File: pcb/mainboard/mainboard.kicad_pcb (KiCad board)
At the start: 2 copper layers, 100 x 100 mm, 50 parts, among them J2 SWD, J3 Conn_01x10, J4 M1, J5 M2, K1 SANYOU_SRD_Form_C, SW1 RES_BUT, SW2 BOOT_SW, U1 STM32G474RETx, U5 INA219AxD, Y1 16MHz

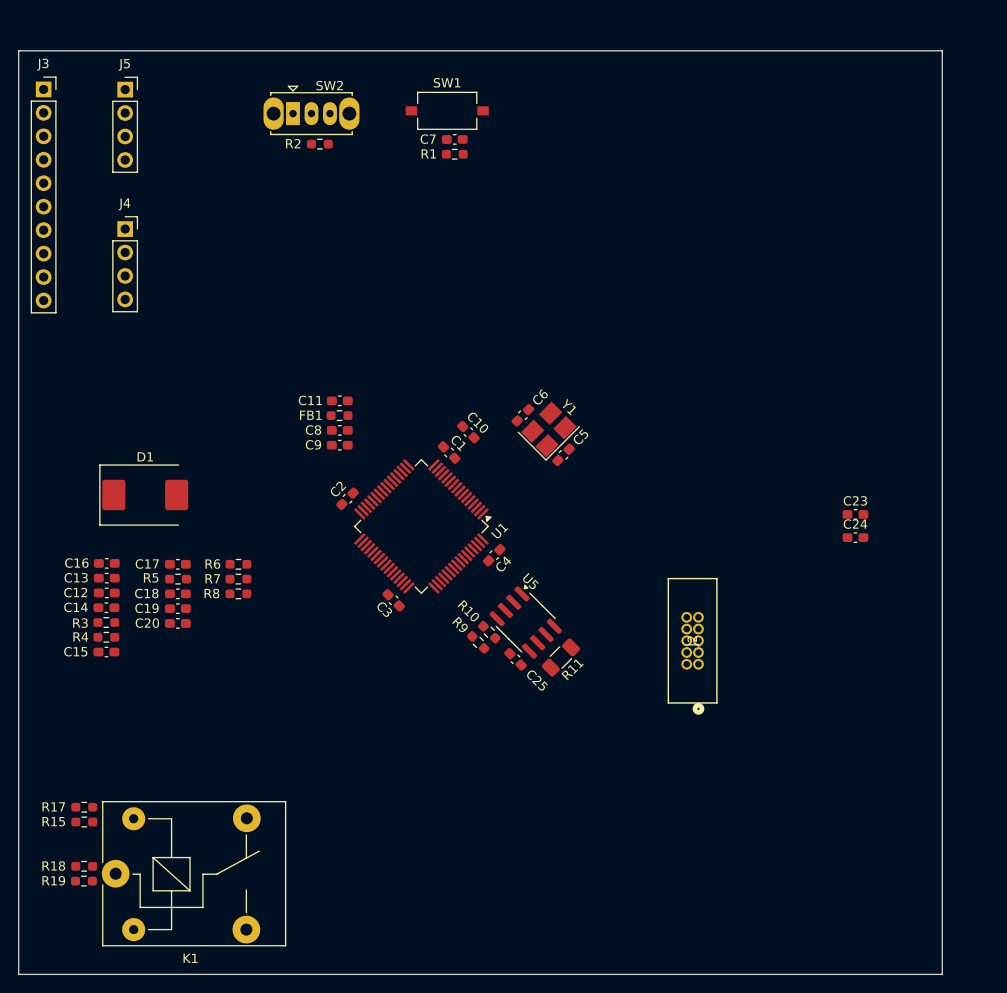
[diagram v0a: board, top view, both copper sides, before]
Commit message: Create pcb
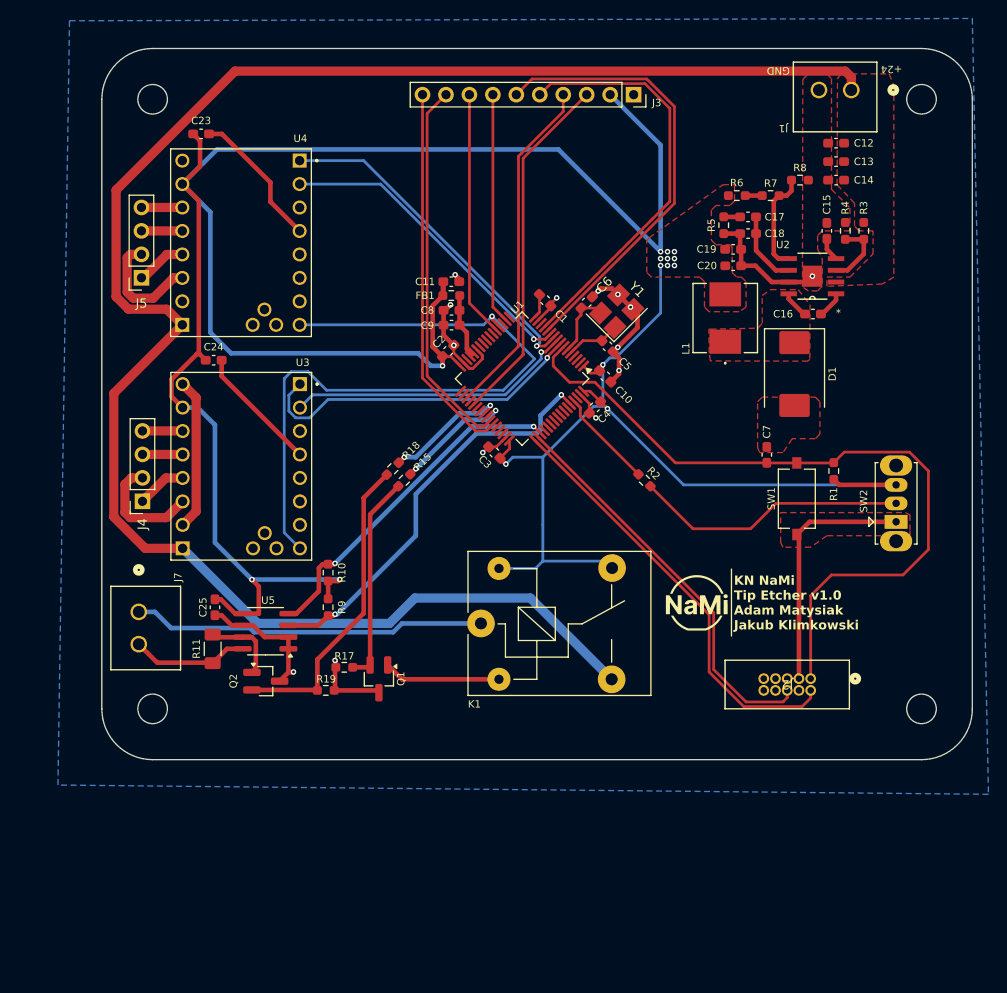
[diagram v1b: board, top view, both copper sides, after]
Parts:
- added G***: LOGO, Graphics:NaMi-logo, F.Cu at (123.4, 82.8)
- added H1: MountingHole, MountingHole:MountingHole_3.2mm_M3, F.Cu at (64.5, 28.2)
- added H2: MountingHole, MountingHole:MountingHole_3.2mm_M3, F.Cu at (147.8, 28.2)
- added H3: MountingHole, MountingHole:MountingHole_3.2mm_M3, F.Cu at (147.8, 94.2)
- added H4: MountingHole, MountingHole:MountingHole_3.2mm_M3, F.Cu at (64.5, 94.2)
- added J1: V_IN, TerminalBlock:CONN_395011002_MOL, F.Cu at (140.1, 27.2)
- added J7: TIP, TerminalBlock:CONN_395011002_MOL, F.Cu at (63.0, 83.8)
- added L1: 6.8u, Inductor_SMD:IND_IHLP-2525CZ_VIS-M, F.Cu at (126.5, 51.9)
- added Q1: NMOS, Package_TO_SOT_SMD:SOT-23_Handsoldering, F.Cu at (89.0, 91.0)
- added Q2: NMOS, Package_TO_SOT_SMD:SOT-23_Handsoldering, F.Cu at (76.8, 91.2)
- added U2: TPS54331DDA, Module:DDA8_3X2P13, F.Cu at (135.9, 47.4)
- added U3: TMC2208_SILENTSTEPSTICK, Connector:MODULE_TMC2208_SILENTSTEPSTICK, F.Cu at (74.1, 68.0)
- added U4: TMC2208_SILENTSTEPSTICK, Connector:MODULE_TMC2208_SILENTSTEPSTICK, F.Cu at (74.1, 43.8)
- moved C12 92.8 mm to (138.5, 33.0), turned to 180 degrees
- moved R3 92.3 mm to (141.5, 42.5), turned to 90 degrees
- moved C14 91.6 mm to (138.5, 37.0), turned to 180 degrees
- moved R4 91.3 mm to (139.5, 42.5), turned to -90 degrees
- moved C13 90.9 mm to (138.5, 35.0), turned to 180 degrees
- moved C15 90.4 mm to (137.5, 42.5), turned to 90 degrees
- moved C23 82.0 mm to (69.8, 32.0)
- moved C16 81.1 mm to (136.0, 51.5)
- moved SW2 78.9 mm to (145.0, 74.0), turned to 90 degrees
- moved R8 75.5 mm to (134.6, 37.0), turned to 180 degrees
- moved C18 73.0 mm to (129.0, 42.8), turned to 180 degrees
- moved C17 72.3 mm to (129.0, 41.0), turned to 180 degrees
- moved C24 72.1 mm to (71.1, 56.5)
- moved C19 71.6 mm to (127.4, 44.5)
- moved C20 71.5 mm to (127.4, 46.3)
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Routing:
- net +3.3V: track 0.00 -> 324.3 mm, vias 0 -> 15
- net +24V: track 0.00 -> 193.9 mm
- net GND: track 0.00 -> 131.1 mm, vias 0 -> 14
- net RESET: track 0.00 -> 81.2 mm
- net M_ENABLE: track 0.00 -> 78.0 mm, vias 0 -> 1
- net OLED_RESET: track 0.00 -> 49.0 mm
- net SWDIO: track 0.00 -> 46.7 mm
- net OLED_DC: track 0.00 -> 45.0 mm
- net INA_SDA: track 0.00 -> 44.8 mm, vias 0 -> 2
- net SWCLK: track 0.00 -> 43.5 mm
- net ENC_SIG_B: track 0.00 -> 41.0 mm
- net ENC_SIG_A: track 0.00 -> 40.6 mm
- net OLED_MOSI: track 0.00 -> 38.6 mm
- net TIP_IN: track 0.00 -> 38.4 mm
- net INA_SCL: track 0.00 -> 37.5 mm, vias 0 -> 2
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- added copper zone on F.Cu, net +24V
- added copper zone on F.Cu, net +3.3V
- added copper zone on B.Cu, net GND
- added copper zone on F.Cu, net GND
- added copper zone on F.Cu, net Net-(D1-K)
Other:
- board size 100 x 100 mm -> 94.2 x 77 mm
- board text added: "+24"
- board text added: "GND"
- board text added: "KN NaMi Tip Etcher v1.0 Adam Matysiak Jakub Klimkowski"
